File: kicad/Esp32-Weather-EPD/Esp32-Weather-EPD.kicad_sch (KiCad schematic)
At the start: 8 parts, among them J2 PINHD_1x4_Female, J3 PINHD_1x8_Male

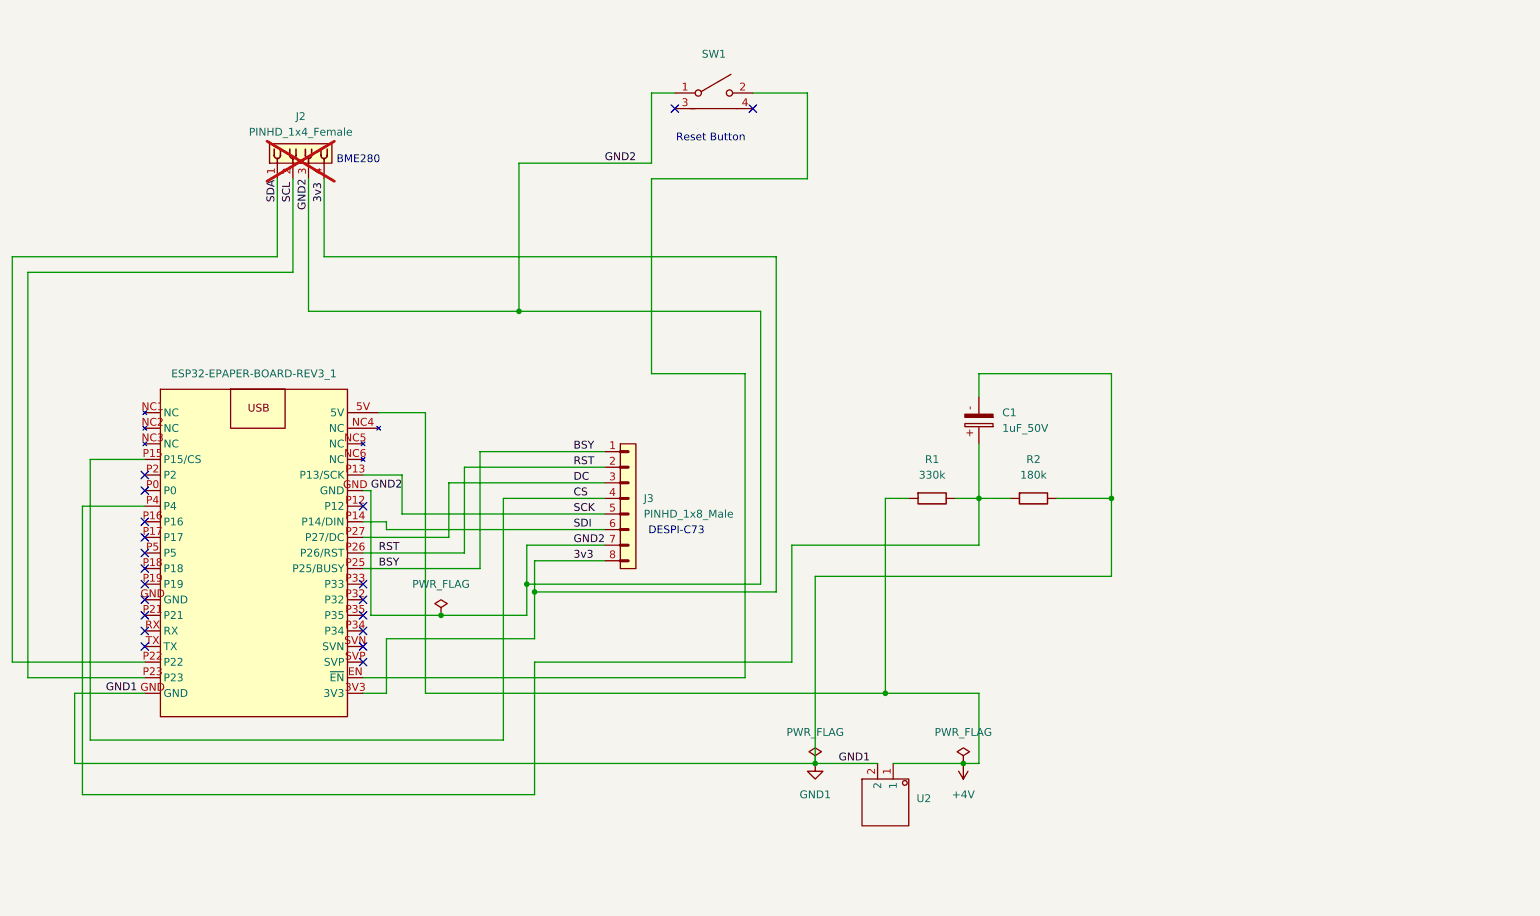
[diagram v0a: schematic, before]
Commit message: kicad
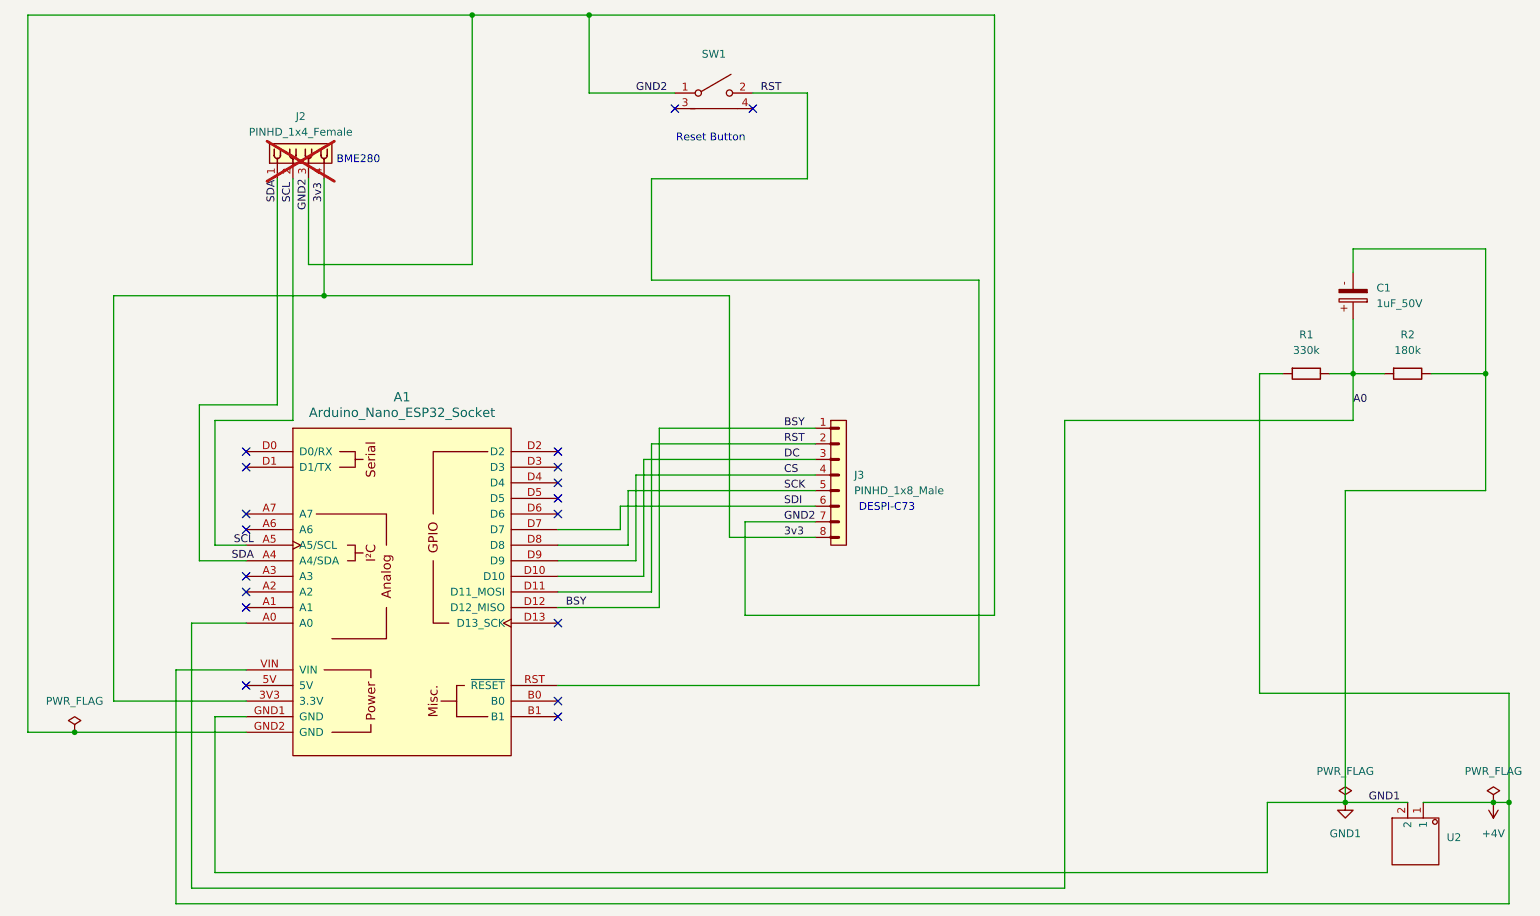
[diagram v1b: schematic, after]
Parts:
- removed ESP32-EPAPER-BOARD-REV3_1: ~, Sephiroth:Waveshare E-Paper Driver Board Rev.3 - ESP32, symbol Waveshare:Waveshare ESP32 E-Paper Driver Board Rev3
- added A1: Arduino_Nano_ESP32_Socket, PCM_arduino-library:Arduino_Nano_ESP32_Socket, symbol PCM_arduino-library:Arduino_Nano_ESP32_Socket
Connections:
- net +4V: now also A1.VIN
- net 3v3: now also A1.3V3 (3.3V)
- net BSY: now also A1.D12 (D12_MISO)
- net CS: now also A1.D9
- net DC: now also A1.D10
- net GND1: now also A1.GND1 (GND)
- net GND2: now also A1.GND2 (GND)
- net RST: now also SW1.2, A1.D11 (D11_MOSI), A1.RST (~{RESET})
- net SCK: now also A1.D8
- net SCL: now also A1.A5 (A5/SCL)
- net SDA: now also A1.A4 (A4/SDA)
- net SDI: now also A1.D7
- net A0: now reaches C1.1, R1.2, R2.1
- net A0: now also A1.A0
- no-connect marks 20 -> 18
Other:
- moved on the sheet: C1, J3, R1, R2, U2
